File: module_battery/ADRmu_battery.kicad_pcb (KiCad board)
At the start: 2 copper layers, 160 x 100 mm, 2 parts, among them J1 Harting 09042326831

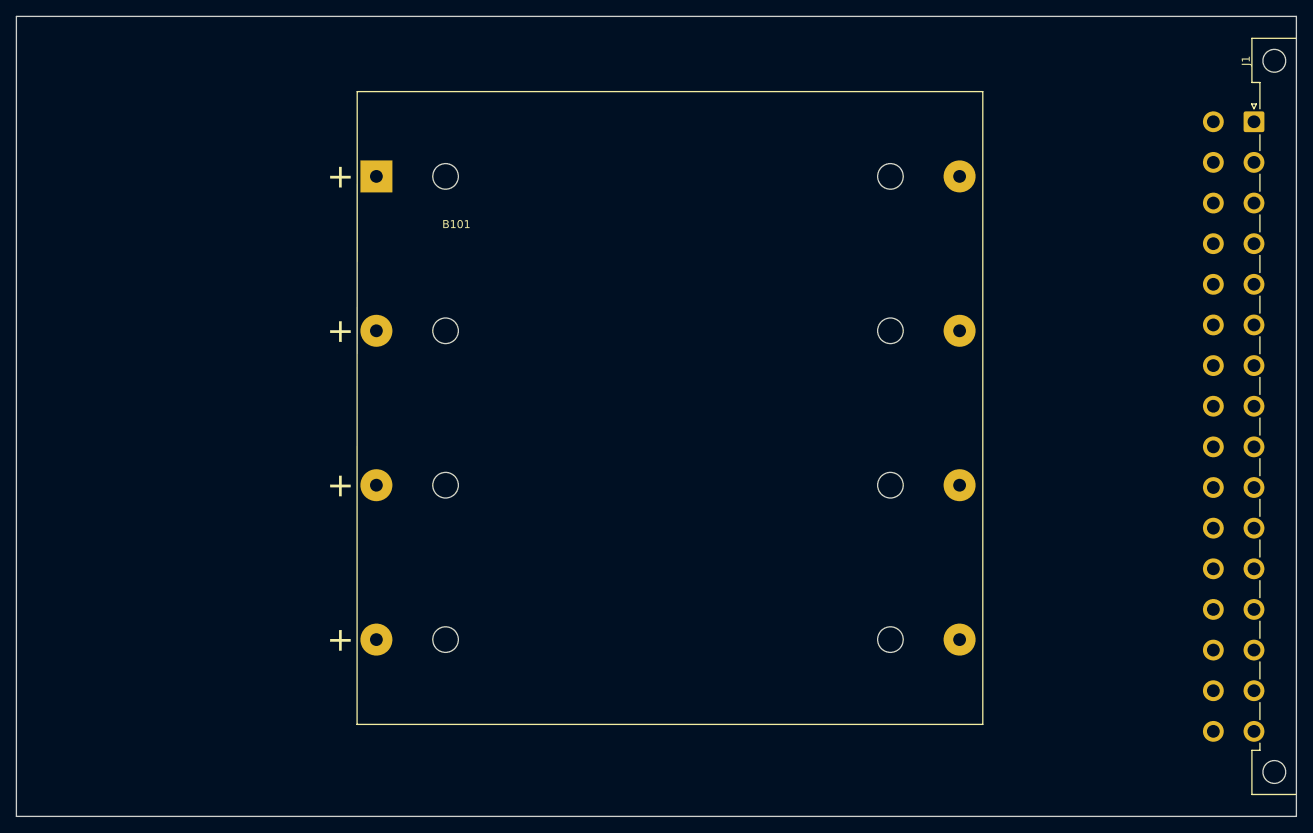
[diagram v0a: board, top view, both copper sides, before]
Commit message: asdf
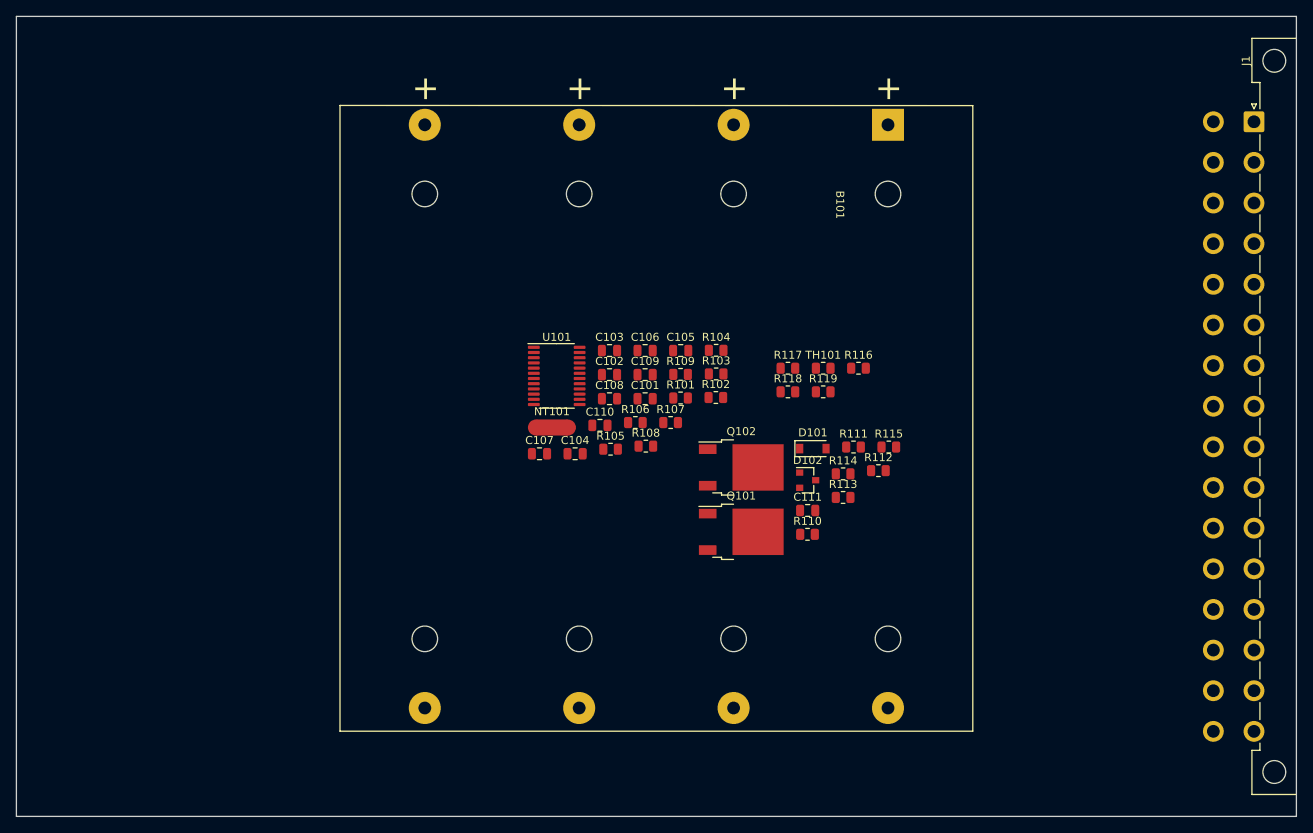
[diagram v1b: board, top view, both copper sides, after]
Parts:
- added C101: 1u 50V, Capacitor_SMD:C_0805_2012Metric, F.Cu at (148.6, 97.8)
- added C102: 1u 50V, Capacitor_SMD:C_0805_2012Metric, F.Cu at (144.1, 94.8)
- added C103: 1u 50V, Capacitor_SMD:C_0805_2012Metric, F.Cu at (144.1, 91.8)
- added C104: 1u 50V, Capacitor_SMD:C_0805_2012Metric, F.Cu at (139.8, 104.7)
- added C105: 1u 50V, Capacitor_SMD:C_0805_2012Metric, F.Cu at (153.0, 91.8)
- added C106: 1u 50V, Capacitor_SMD:C_0805_2012Metric, F.Cu at (148.6, 91.8)
- added C107: 1u 50V, Capacitor_SMD:C_0805_2012Metric, F.Cu at (135.4, 104.7)
- added C108: 100n 50V, Capacitor_SMD:C_0805_2012Metric, F.Cu at (144.1, 97.8)
- added C109: 100n 50V, Capacitor_SMD:C_0805_2012Metric, F.Cu at (148.6, 94.8)
- added C110: 100n 50V, Capacitor_SMD:C_0805_2012Metric, F.Cu at (142.9, 101.1)
- added C111: 100n 50V, Capacitor_SMD:C_0805_2012Metric, F.Cu at (168.9, 111.8)
- added D101: 1N4148, Diode_SMD:D_SOD-123, F.Cu at (169.6, 104.0)
- added D102: 16V, Diode_SMD:D_SOT-23_ANK, F.Cu at (168.9, 108.0)
- added NT101: NetTie_2, NetTie:NetTie-2_SMD_Pad2.0mm, F.Cu at (136.9, 101.4)
- added Q101: Q_NMOS_GDS, Package_TO_SOT_SMD:TO-252-2, F.Cu at (160.6, 114.4)
- added Q102: Q_NMOS_GDS, Package_TO_SOT_SMD:TO-252-2, F.Cu at (160.6, 106.4)
- added R101: 1k, Resistor_SMD:R_0805_2012Metric, F.Cu at (153.0, 97.7)
- added R102: 47, Resistor_SMD:R_0805_2012Metric, F.Cu at (157.4, 97.6)
- added R103: 47, Resistor_SMD:R_0805_2012Metric, F.Cu at (157.5, 94.7)
- added R104: 47, Resistor_SMD:R_0805_2012Metric, F.Cu at (157.5, 91.7)
- added R105: 47, Resistor_SMD:R_0805_2012Metric, F.Cu at (144.3, 104.1)
- added R106: 47, Resistor_SMD:R_0805_2012Metric, F.Cu at (147.4, 100.8)
- added R107: 100, Resistor_SMD:R_0805_2012Metric, F.Cu at (151.8, 100.8)
- added R108: 1, Resistor_SMD:R_0805_2012Metric, F.Cu at (148.7, 103.7)
- added R109: 100, Resistor_SMD:R_0805_2012Metric, F.Cu at (153.0, 94.8)
- added R110: 5k1, Resistor_SMD:R_0805_2012Metric, F.Cu at (168.9, 114.7)
- added R111: 10M, Resistor_SMD:R_0805_2012Metric, F.Cu at (174.6, 103.8)
- added R112: 5k1, Resistor_SMD:R_0805_2012Metric, F.Cu at (177.8, 106.8)
- added R113: 3M, Resistor_SMD:R_0805_2012Metric, F.Cu at (173.3, 110.1)
- added R114: 470k, Resistor_SMD:R_0805_2012Metric, F.Cu at (173.3, 107.2)
- added R115: 1M, Resistor_SMD:R_0805_2012Metric, F.Cu at (179.1, 103.8)
- added R116: 10k, Resistor_SMD:R_0805_2012Metric, F.Cu at (175.3, 94.0)
- added R117: 200k, Resistor_SMD:R_0805_2012Metric, F.Cu at (166.4, 94.0)
- added R118: 10k, Resistor_SMD:R_0805_2012Metric, F.Cu at (166.4, 96.9)
- added R119: 10k, Resistor_SMD:R_0805_2012Metric, F.Cu at (170.8, 96.9)
- added TH101: Thermistor_NTC, Resistor_SMD:R_0805_2012Metric, F.Cu at (170.8, 94.0)
- added U101: BQ77915, Package_SO:TSSOP-24_4.4x7.8mm_P0.65mm, F.Cu at (137.5, 94.9)
- moved B101 64.3 mm to (178.9, 63.5), turned to -90 degrees
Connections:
- B101 pad 1: unconnected-(B101-Pad1) -> +BATT
- B101 pad 8: unconnected-(B101-Pad8) -> -BATT
